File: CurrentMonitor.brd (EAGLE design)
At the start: 83 x 100 mm, 68 parts, among them IC1 MEGA8-AI, IC2 INA138, IC3 INA138, IC4 LF33CV, J1 AVR_SPI_PRG_6OFFSET_PADS, Q1 10MHz, Q2 IRLZ34N, Q3 IRLZ34N, Q4 IRLZ34N, Q6 BC847, Q7 IRF9530, Q8 IRF9530, Q9 BC847, X1 MSTBV2, X2 MSTBV2, X3 MSTBV2, X5 MSTBV2

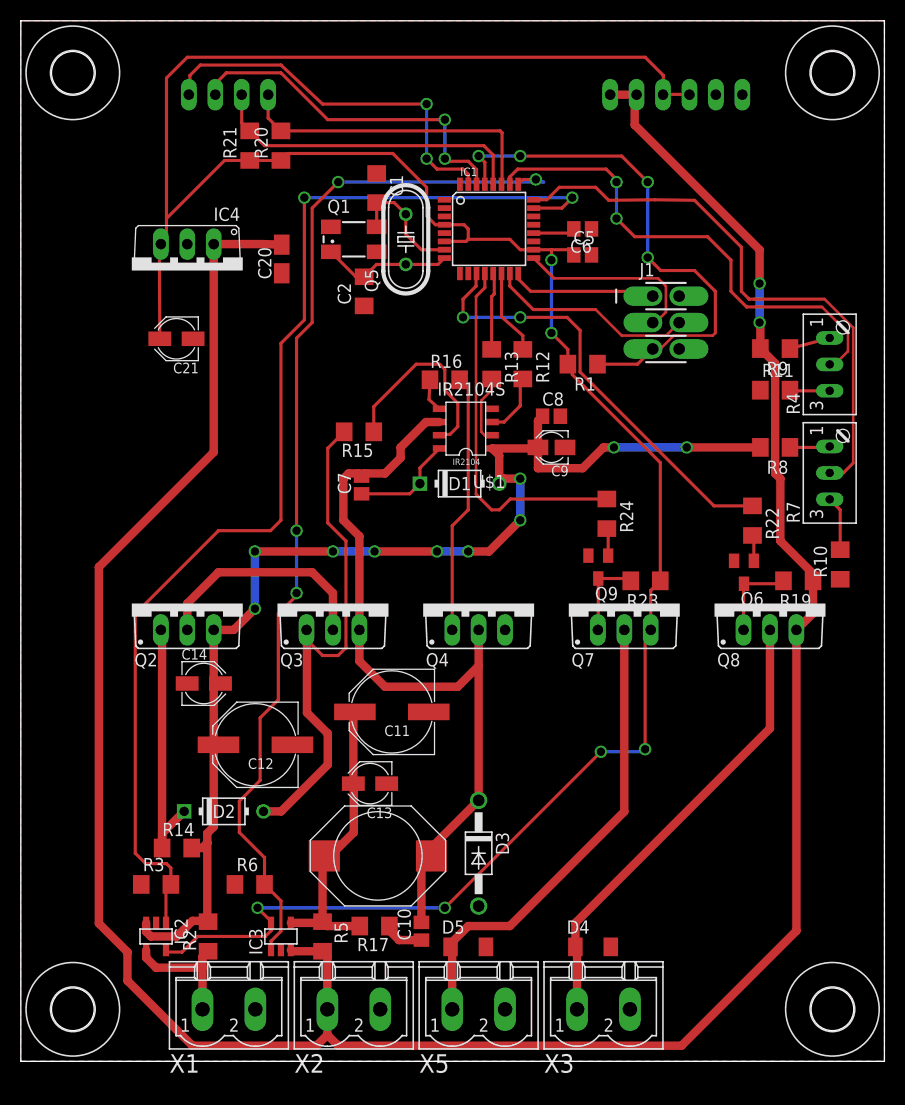
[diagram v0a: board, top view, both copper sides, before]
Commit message: Second revision, dual layer
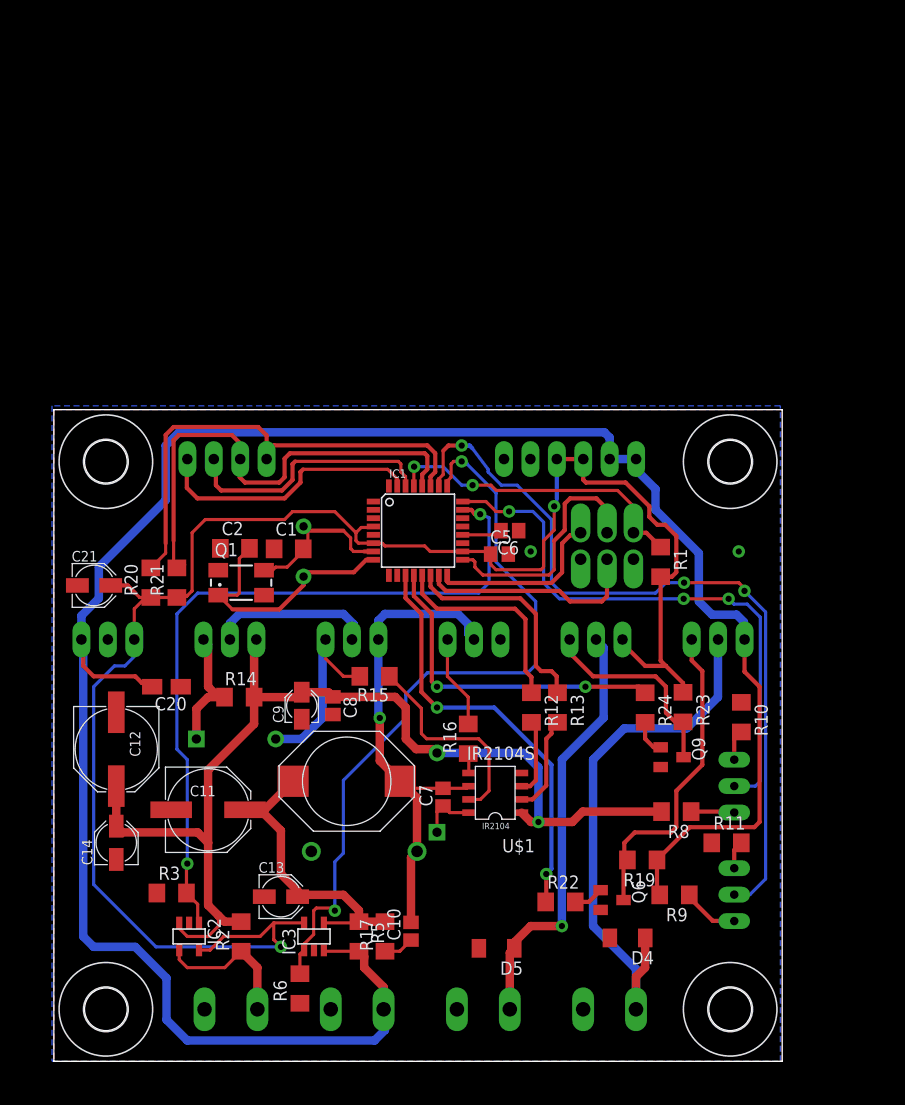
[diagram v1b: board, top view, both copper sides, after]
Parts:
- moved R9 53.4 mm to (59.8, 16.0)
- moved R4 51.8 mm to (66.8, 16.0), flipped to the bottom, turned to 270 degrees
- moved R20 43.8 mm to (9.50, 46.0)
- moved R11 43.8 mm to (64.8, 21.0)
- moved R21 42.6 mm to (12.0, 46.0)
- moved C20 42.6 mm to (11.0, 36.0), turned to 180 degrees
- moved R22 41.0 mm to (48.9, 15.3), turned to 0 degrees
- moved IC4 38.8 mm to (5.37, 38.0), flipped to the bottom
- moved U$5 38.6 mm to (65.2, 57.6)
- moved U$3 37.5 mm to (5.17, 57.6)
- moved JP1 36.5 mm to (49.8, 57.9), turned to 180 degrees
- moved R8 36.3 mm to (60.0, 24.0)
- moved C1 35.7 mm to (22.7, 49.3), turned to 0 degrees
- moved U$1 35.1 mm to (45.1, 27.7)
- moved JP2 35.0 mm to (16.8, 57.9)
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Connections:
- net MPPT_ENABLE: now also IC1.13; no longer IC1.14
- net MPPT_PWM: now also IC1.14; no longer IC1.13
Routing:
- net +3V3: track 239.7 -> 169.7 mm, vias 6 -> 2
- net BAT+: track 257.4 -> 212.5 mm, vias 2 -> 0
- net ADC0: track 112.0 -> 70.9 mm
- net N$13: track 49.6 -> 18.8 mm
- net ADC2: track 102.2 -> 72.2 mm, vias 4 -> 2
- net ADC3: track 48.0 -> 75.5 mm, vias 2 -> 3
- net VS: track 74.3 -> 47.8 mm, vias 0 -> 1
- net N$20: track 8.37 -> 30.9 mm
- net RESET: track 51.9 -> 30.2 mm, vias 4 -> 2
- net SDA: track 30.3 -> 46.7 mm
- net N$11: track 25.1 -> 8.95 mm
- net SCL: track 31.0 -> 47.1 mm
- net CELL_TO_CONTROLLER: track 117.7 -> 102.4 mm, vias 10 -> 1
- net MPPT_PWM: track 7.43 -> 21.3 mm
- net N$12: track 25.4 -> 12.8 mm
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- added copper zone on layer 16, net GND
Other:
- board size 83 x 100 mm -> 70 x 62.6 mm
